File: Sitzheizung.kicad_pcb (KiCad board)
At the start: 2 copper layers, 1 part, among them Q1 BUK9M9R1-40EX

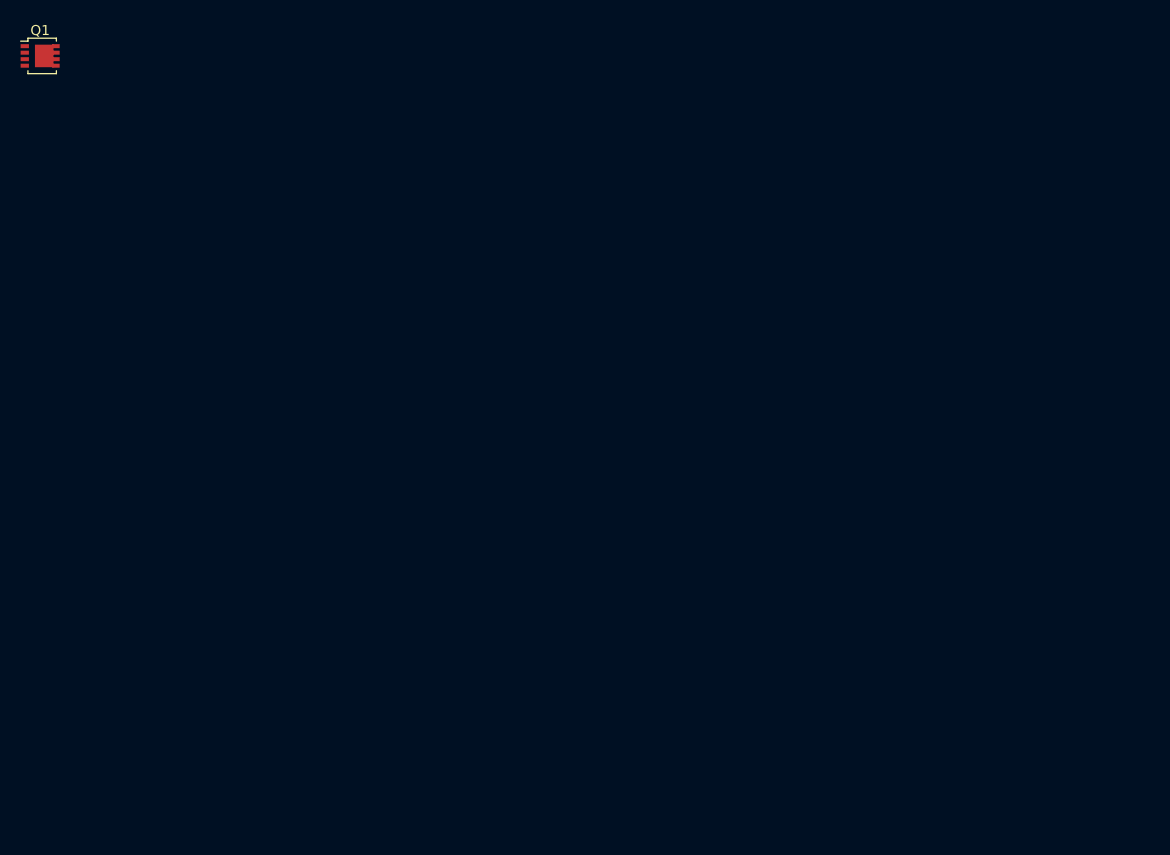
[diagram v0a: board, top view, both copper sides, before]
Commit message: finished layout
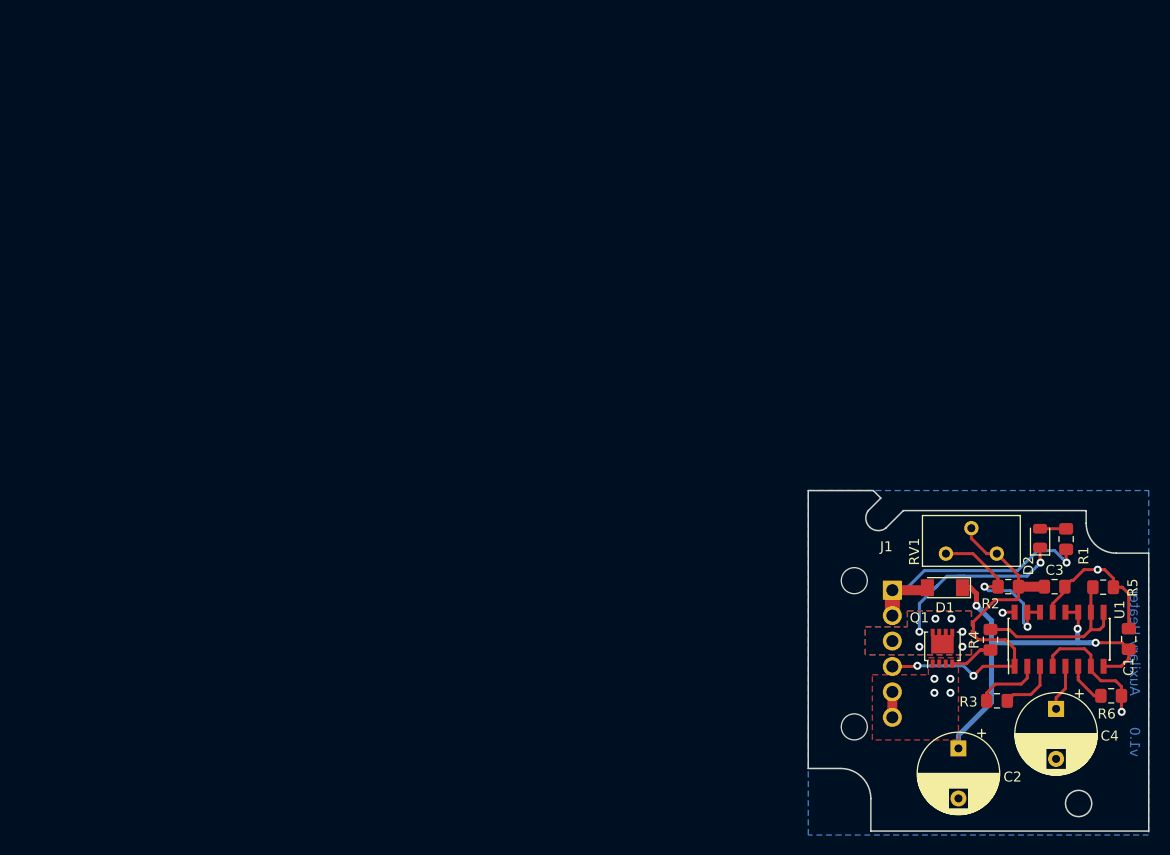
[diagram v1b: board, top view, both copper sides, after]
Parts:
- added C1: 100n, Capacitor_SMD:C_0805_2012Metric_Pad1.15x1.40mm_HandSolder, F.Cu at (163.5, 102.8)
- added C2: 10u, Capacitor_THT:CP_Radial_D8.0mm_P5.00mm, F.Cu at (146.5, 113.8)
- added C3: 100n, Capacitor_SMD:C_0805_2012Metric_Pad1.15x1.40mm_HandSolder, F.Cu at (156.1, 97.6)
- added C4: 1u, Capacitor_THT:CP_Radial_D8.0mm_P5.00mm, F.Cu at (156.2, 109.8)
- added D1: D, Diode_SMD:D_MiniMELF, F.Cu at (145.2, 97.7)
- added D2: LED, LED_SMD:LED_0805_2012Metric_Pad0.98x1.40mm_HandSolder, F.Cu at (154.7, 92.8)
- added J1: Conn_01x06_Male, Connector_TE-Connectivity:TE_MQS_936287-2_1x06_P2.54mm_Horizontal, F.Cu at (139.9, 98.0)
- added R1: 650R, Resistor_SMD:R_0805_2012Metric_Pad1.15x1.40mm_HandSolder, F.Cu at (157.2, 92.8)
- added R2: R, Resistor_SMD:R_0805_2012Metric_Pad1.15x1.40mm_HandSolder, F.Cu at (151.5, 97.6)
- added R3: 1k, Resistor_SMD:R_0805_2012Metric_Pad1.15x1.40mm_HandSolder, F.Cu at (150.3, 109.0)
- added R4: 15k, Resistor_SMD:R_0805_2012Metric_Pad1.15x1.40mm_HandSolder, F.Cu at (149.7, 102.9)
- added R5: 1k8, Resistor_SMD:R_0805_2012Metric_Pad1.15x1.40mm_HandSolder, F.Cu at (160.9, 97.7)
- added R6: 1k, Resistor_SMD:R_0805_2012Metric_Pad1.15x1.40mm_HandSolder, F.Cu at (161.8, 108.5)
- added RV1: 15k, Potentiometer_THT:Potentiometer_Bourns_3386X_Horizontal, F.Cu at (145.2, 94.3)
- added U1: TL494, Package_SO:SOIC-16_3.9x9.9mm_P1.27mm, F.Cu at (156.6, 102.8)
- moved Q1 107.8 mm to (144.9, 103.8), turned to 90 degrees
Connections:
- Q1 pad 4: (no net) -> Net-(Q1-Pad4)
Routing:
- net Net-(C1-Pad1): track 0.00 -> 41.9 mm, vias 0 -> 3
- net Poti_1: track 0.00 -> 38.3 mm, vias 0 -> 2
- net KL31: track 0.00 -> 32.1 mm, vias 0 -> 7
- net Heizung+: track 0.00 -> 27.0 mm, vias 0 -> 1
- net Heizung-: track 0.00 -> 19.1 mm, vias 0 -> 7
- net Net-(R2-Pad1): track 0.00 -> 18.2 mm, vias 0 -> 2
- net Net-(R4-Pad2): track 0.00 -> 17.7 mm
- net Net-(R3-Pad1): track 0.00 -> 6.64 mm
- net Net-(R3-Pad2): track 0.00 -> 5.81 mm
- net Net-(C4-Pad1): track 0.00 -> 4.64 mm
- net Net-(Q1-Pad4): track 0.00 -> 4.62 mm
- net Net-(R6-Pad1): track 0.00 -> 4.29 mm
- net Net-(D2-Pad2): track 0.00 -> 2.61 mm
- added copper zone on B.Cu, net Heizung-
- added copper zone on F.Cu, net Heizung-
- added copper zone on B.Cu, net KL31
- added copper zone on F.Cu, net KL31
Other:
- board outline added: 34 x 34 mm
- net class Default: clearance 0.2 -> 0.15
- rule trace_clearance: 0.2 -> 0.15
- rule trace_min: 0.2 -> 0.15
- board text added: "Auxilary Heater"
- board text added: "v1.0"
